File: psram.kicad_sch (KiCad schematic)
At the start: 5 parts

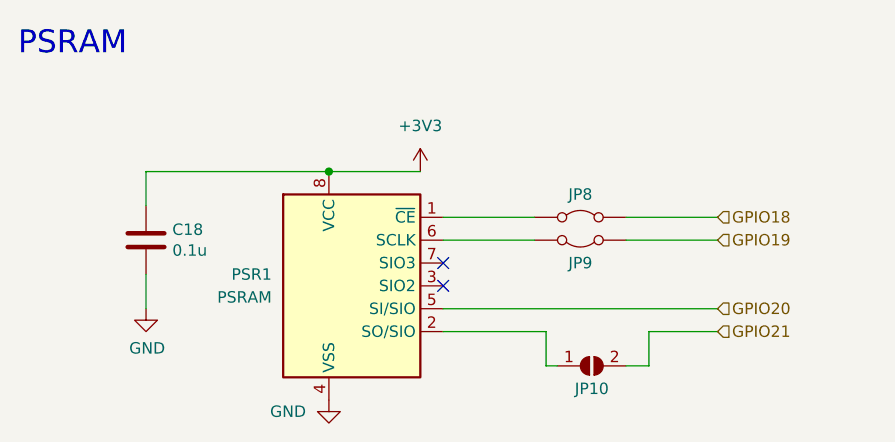
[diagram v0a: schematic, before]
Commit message: WIP
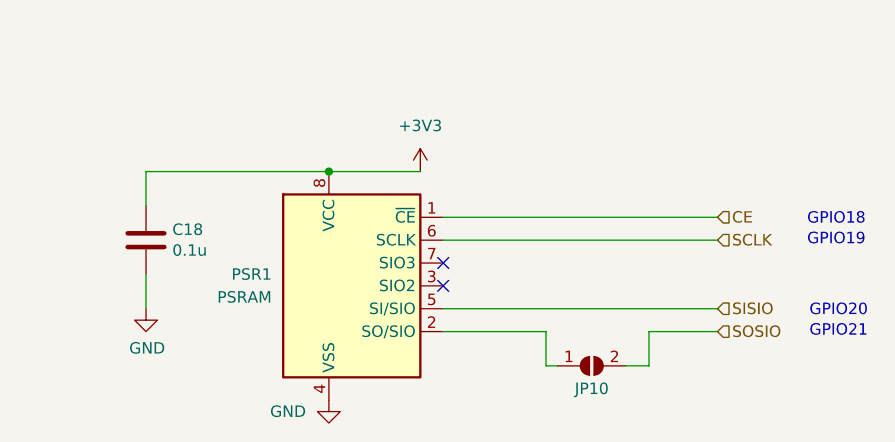
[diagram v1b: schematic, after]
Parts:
- removed JP8, JP9: RP ZERO +5V Jumper, LIBS:Medved_PinHeader_1x02_P2.54mm_Vertical_R, symbol Jumper:Jumper_2_Bridged
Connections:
- net CE: now reaches PSR1.1 (~{CE})
- net SCLK: now reaches PSR1.6 (SCLK)
- net GPIO20 renamed SISIO
- net GPIO21 renamed SOSIO
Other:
- note added: "GPIO18"
- note added: "GPIO19"
- note added: "GPIO20"
- note added: "GPIO21"
- note removed: "PSRAM"
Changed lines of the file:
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@@
 	(wire
 		(pts
-			(xy 74.93 45.72) (xy 85.09 45.72)
-		)
-		(stroke
-			(width 0)
-			(type default)
-		)
-	)
-	(wire
-		(pts
-			(xy 95.25 48.26) (xy 105.41 48.26)
-		)
-		(stroke
-			(width 0)
-			(type default)
-		)
-	)
-	(wire
-		(pts
-			(xy 95.25 45.72) (xy 105.41 45.72)
+			(xy 74.93 45.72) (xy 105.41 45.72)
 		)
 		(stroke
@@
 	(wire
 		(pts
-			(xy 74.93 48.26) (xy 85.09 48.26)
+			(xy 74.93 48.26) (xy 105.41 48.26)
 		)
 		(stroke
@@
 		)
 	)
-	(text "PSRAM"
-		(exclude_from_sim no)
-		(at 27.686 27.94 0)
-		(effects
-			(font
-				(size 2.54 2.54)
-			)
-			(justify left bottom)
-		)
-	)
-	(hierarchical_label "GPIO20"
+	(text "GPIO21"
+		(exclude_from_sim no)
+		(at 118.872 58.42 0)
+		(effects
+			(font
+				(size 1.27 1.27)
+			)
+		)
+	)
+	(text "GPIO19"
+		(exclude_from_sim no)
+		(at 118.618 48.26 0)
+		(effects
+			(font
+				(size 1.27 1.27)
+			)
+		)
+	)
+	(text "GPIO20"
+		(exclude_from_sim no)
+		(at 118.872 56.134 0)
+		(effects
+			(font
+				(size 1.27 1.27)
+			)
+		)
+	)
+	(text "GPIO18"
+		(exclude_from_sim no)
+		(at 118.618 45.974 0)
+		(effects
+			(font
+				(size 1.27 1.27)
+			)
+		)
+	)
+	(hierarchical_label "SISIO"
 		(shape input)
 		(at 105.41 55.88 0)
@@
 		)
 	)
-	(hierarchical_label "GPIO18"
+	(hierarchical_label "CE"
 		(shape input)
 		(at 105.41 45.72 0)
@@
 		)
 	)
-	(hierarchical_label "GPIO19"
+	(hierarchical_label "SCLK"
 		(shape input)
 		(at 105.41 48.26 0)
@@
 		)
 	)
-	(hierarchical_label "GPIO21"
+	(hierarchical_label "SOSIO"
 		(shape input)
 		(at 105.41 58.42 0)
@@
 			)
 			(justify left)
-		)
-	)
-	(symbol
-		(lib_id "Jumper:Jumper_2_Bridged")
-		(at 90.17 45.72 0)
-		(unit 1)
-		(exclude_from_sim yes)
-		(in_bom yes)
-		(on_board yes)
-		(dnp no)
-		(property "Reference" "JP8"
-			(at 90.17 43.18 0)
-			(effects
-				(font
-					(size 1.27 1.27)
-				)
-			)
-		)
-		(property "Value" "RP ZERO +5V Jumper"
-			(at 90.17 43.18 0)
-			(effects
-				(font
-					(size 1.27 1.27)
-				)
-				(hide yes)
-			)
-		)
-		(property "Footprint" "LIBS:Medved_PinHeader_1x02_P2.54mm_Vertical_R"
-			(at 90.17 45.72 0)
-			(effects
-				(font
-					(size 1.27 1.27)
-				)
-				(hide yes)
-			)
-		)
-		(property "Datasheet" "~"
-			(at 90.17 45.72 0)
-			(effects
-				(font
-					(size 1.27 1.27)
-				)
-				(hide yes)
-			)
-		)
-		(property "Description" "Jumper, 2-pole, closed/bridged"
-			(at 90.17 45.72 0)
-			(effects
-				(font
-					(size 1.27 1.27)
-				)
-				(hide yes)
-			)
-		)
-		(pin "2"
-		)
-		(pin "1"
-		)
-		(instances
-			(project "frank2"
-				(path "/8c0b3d8b-46d3-4173-ab1e-a61765f77d61/cfde7a60-7ac3-405d-8b86-f95521b6825b"
-					(reference "JP8")
-					(unit 1)
-				)
-			)
 		)
 	)
@@
 		(instances
 			(project "frank2"
-				(path "/8c0b3d8b-46d3-4173-ab1e-a61765f77d61/cfde7a60-7ac3-405d-8b86-f95521b6825b"
-					(reference "#PWR045")
-					(unit 1)
-				)
-			)
-		)
-	)
-	(symbol
-		(lib_id "Jumper:Jumper_2_Bridged")
-		(at 90.17 48.26 180)
-		(unit 1)
-		(exclude_from_sim yes)
-		(in_bom yes)
-		(on_board yes)
-		(dnp no)
-		(property "Reference" "JP9"
-			(at 90.17 50.8 0)
-			(effects
-				(font
-					(size 1.27 1.27)
-				)
-			)
-		)
-		(property "Value" "RP ZERO +5V Jumper"
-			(at 90.17 50.8 0)
-			(effects
-				(font
-					(size 1.27 1.27)
-				)
-				(hide yes)
-			)
-		)
-		(property "Footprint" "LIBS:Medved_PinHeader_1x02_P2.54mm_Vertical_R"
-			(at 90.17 48.26 0)
-			(effects
-				(font
-					(size 1.27 1.27)
-				)
-				(hide yes)
-			)
-		)
-		(property "Datasheet" "~"
-			(at 90.17 48.26 0)
-			(effects
-				(font
-					(size 1.27 1.27)
-				)
-				(hide yes)
-			)
-		)
-		(property "Description" "Jumper, 2-pole, closed/bridged"
-			(at 90.17 48.26 0)
-			(effects
-				(font
-					(size 1.27 1.27)
-				)
-				(hide yes)
-			)
-		)
-		(pin "2"
-		)
-		(pin "1"
-		)
-		(instances
-			(project "frank2"
-				(path "/8c0b3d8b-46d3-4173-ab1e-a61765f77d61/cfde7a60-7ac3-405d-8b86-f95521b6825b"
-					(reference "JP9")
+				(path "/8c0b3d8b-46d3-4173-ab1e-a61765f77d61/c6465a8b-a48e-459c-b6f3-7a504929a2d8"
+					(reference "#PWR055")
 					(unit 1)
 				)
@@
 		(instances
 			(project ""
-				(path "/8c0b3d8b-46d3-4173-ab1e-a61765f77d61/cfde7a60-7ac3-405d-8b86-f95521b6825b"
-					(reference "#PWR067")
+				(path "/8c0b3d8b-46d3-4173-ab1e-a61765f77d61/c6465a8b-a48e-459c-b6f3-7a504929a2d8"
+					(reference "#PWR056")
 					(unit 1)
 				)
@@
 		(instances
 			(project "frank2"
-				(path "/8c0b3d8b-46d3-4173-ab1e-a61765f77d61/cfde7a60-7ac3-405d-8b86-f95521b6825b"
+				(path "/8c0b3d8b-46d3-4173-ab1e-a61765f77d61/c6465a8b-a48e-459c-b6f3-7a504929a2d8"
 					(reference "PSR1")
 					(unit 1)
@@
 		(instances
 			(project "frank2"
-				(path "/8c0b3d8b-46d3-4173-ab1e-a61765f77d61/cfde7a60-7ac3-405d-8b86-f95521b6825b"
-					(reference "C18")
+				(path "/8c0b3d8b-46d3-4173-ab1e-a61765f77d61/c6465a8b-a48e-459c-b6f3-7a504929a2d8"
+					(reference "C25")
 					(unit 1)
 				)
@@
 		(instances
 			(project "frank2"
-				(path "/8c0b3d8b-46d3-4173-ab1e-a61765f77d61/cfde7a60-7ac3-405d-8b86-f95521b6825b"
-					(reference "JP10")
+				(path "/8c0b3d8b-46d3-4173-ab1e-a61765f77d61/c6465a8b-a48e-459c-b6f3-7a504929a2d8"
+					(reference "JP3")
 					(unit 1)
 				)
@@
 		(instances
 			(project "frank2"
-				(path "/8c0b3d8b-46d3-4173-ab1e-a61765f77d61/cfde7a60-7ac3-405d-8b86-f95521b6825b"
-					(reference "#PWR044")
+				(path "/8c0b3d8b-46d3-4173-ab1e-a61765f77d61/c6465a8b-a48e-459c-b6f3-7a504929a2d8"
+					(reference "#PWR054")
 					(unit 1)
 				)
